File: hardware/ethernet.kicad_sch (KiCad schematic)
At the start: 3 parts, among them J1 RJ45_Hanrun_HR911105A_Horizon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

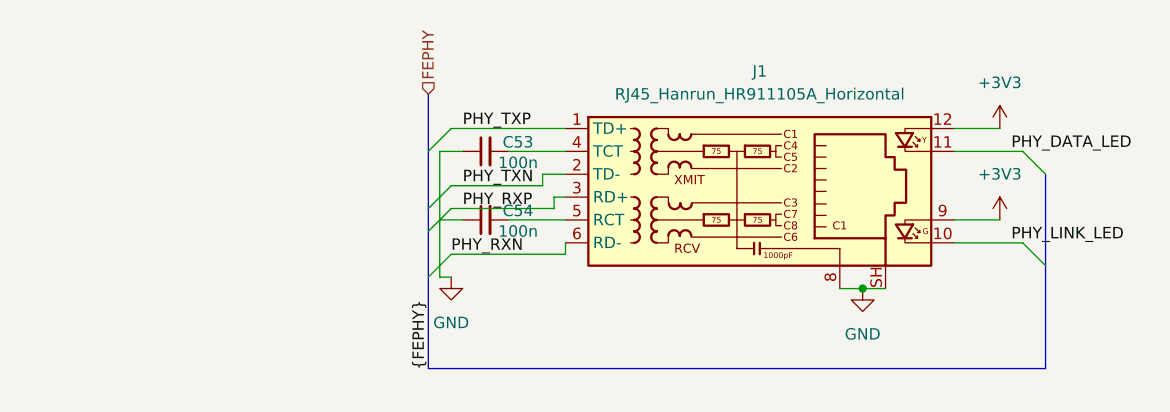
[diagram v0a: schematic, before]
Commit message: final touches
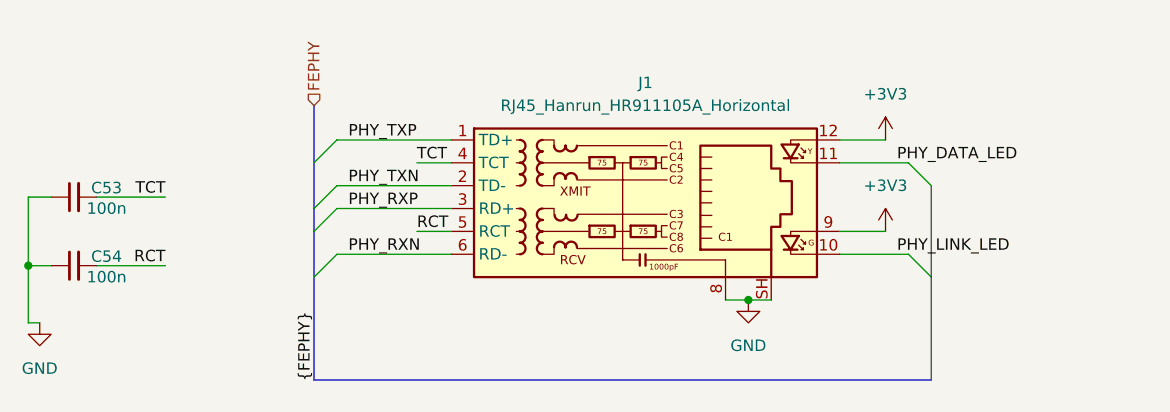
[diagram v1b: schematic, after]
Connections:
- net RCT: now reaches C54.2, J1.5 (RCT)
- net TCT: now reaches C53.2, J1.4 (TCT)
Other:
- moved on the sheet: J1
